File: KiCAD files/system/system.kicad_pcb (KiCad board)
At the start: 2 copper layers, 96.5 x 71.1 mm, 16 parts, among them J1 Input, J2 Conn_01x04_Female, SW1 SW_Push, U1 ATmega328P-P, Y1 Crystal

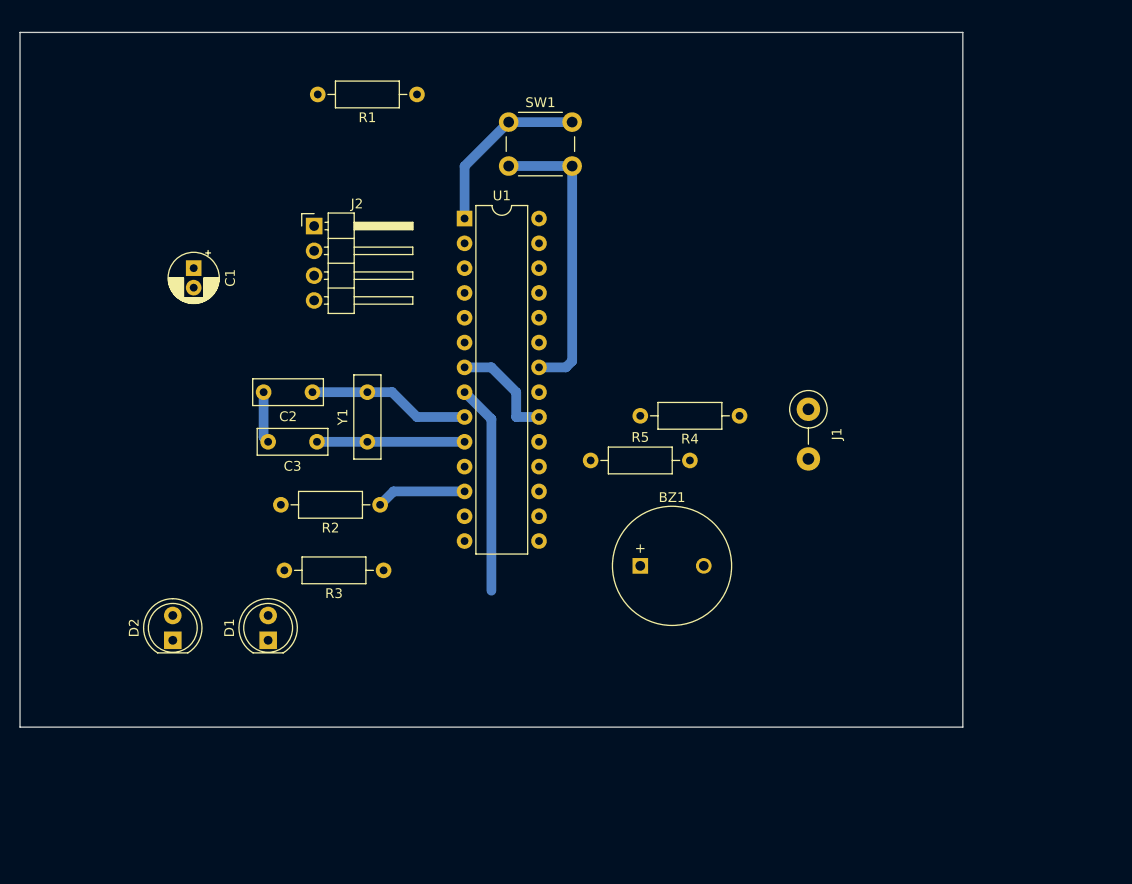
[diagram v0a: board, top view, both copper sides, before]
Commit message: edited system pcb
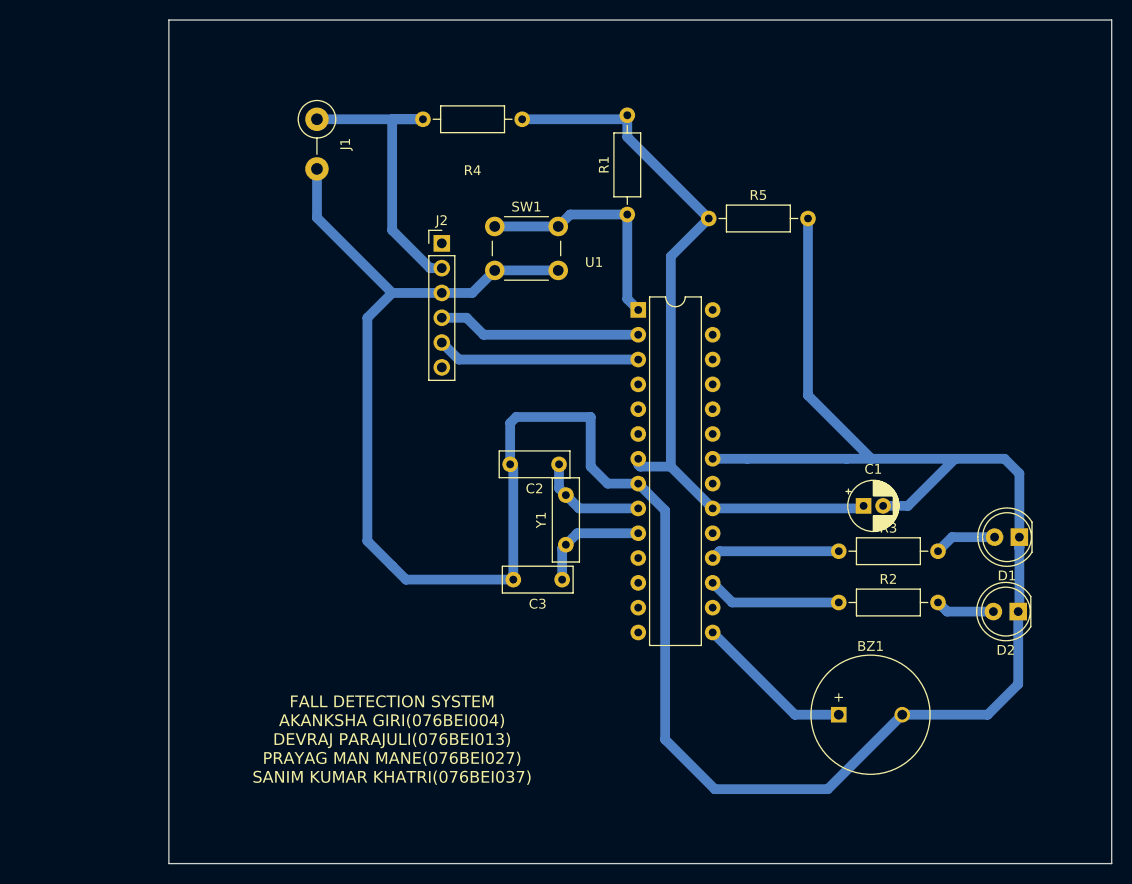
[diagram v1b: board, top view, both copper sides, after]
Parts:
- C1: value C_Polarized -> 10u
- J2: value Conn_01x04_Female -> Conn_01x06_Female; footprint Connector_PinHeader_2.54mm:PinHeader_1x04_P2.54mm_Horizontal -> Connector_PinHeader_2.54mm:PinHeader_1x06_P2.54mm_Vertical
- R1: value R -> 10k
- R2, R3: value R -> 440
- moved D2 86.6 mm to (196.2, 108.8), turned to 180 degrees
- moved D1 77.6 mm to (196.3, 101.2), turned to 180 degrees
- moved C1 72.8 mm to (180.3, 98.0), turned to 0 degrees
- moved J1 58.4 mm to (124.4, 58.4)
- moved R2 48.0 mm to (177.8, 107.9), turned to 0 degrees
- moved R3 46.6 mm to (177.8, 102.6), turned to 0 degrees
- moved R4 44.4 mm to (135.2, 58.4), turned to 0 degrees
- moved C3 28.8 mm to (149.5, 105.5)
- moved R5 27.6 mm to (164.5, 68.6)
- moved C2 26.3 mm to (149.2, 93.7)
- moved BZ1 25.4 mm to (177.8, 119.4)
- moved R1 24.8 mm to (156.2, 68.2), turned to 90 degrees
- moved Y1 22.9 mm to (149.9, 102.0)
- moved U1 20.1 mm to (157.3, 77.9)
- moved J2 13.2 mm to (137.2, 71.1)
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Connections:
- J2 pad 1: +3.3V -> unconnected-(J2-Pad1)
- J2 pad 2: /data -> +5V
- J2 pad 3: /data -> GND
- J2 pad 4: GND -> /txd
- U1 pad 12: /PD6 -> unconnected-(U1-Pad12)
- U1 pad 13: /PD7 -> unconnected-(U1-Pad13)
- U1 pad 17: unconnected-(U1-Pad17) -> /PD6
- U1 pad 18: unconnected-(U1-Pad18) -> /PD7
- U1 pad 2: /data -> /txd
- U1 pad 3: unconnected-(U1-Pad3) -> /rxd
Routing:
- net GND: track 56.9 -> 273.6 mm
- net +3.3V: track 11.2 -> 77.6 mm
- net +5V: track 0.00 -> 32.0 mm
- net /txd: track 0.00 -> 20.8 mm
- net /rxd: track 0.00 -> 20.8 mm
- net /PB1: track 0.00 -> 16.4 mm
- net /PD7: track 0.21 -> 13.2 mm
- net Net-(D1-Pad2): track 0.00 -> 6.39 mm
- net Net-(D2-Pad2): track 0.00 -> 6.06 mm
- net Net-(R1-Pad1): track 18.7 -> 24.3 mm
- net Net-(C2-Pad1): track 16.6 -> 11.4 mm
- net /PD6: track 9.21 -> 13.7 mm
- net Net-(C3-Pad1): track 15.1 -> 11.6 mm
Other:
- board size 96.5 x 71.1 mm -> 96.5 x 86.4 mm
- board text added: "FALL DETECTION SYSTEM AKANKSHA GIRI(076BEI004) DEVRAJ PARAJULI(076BEI013) PRAYAG MAN MANE(076BEI027) SANIM KUMAR KHATRI(076BEI037)"
